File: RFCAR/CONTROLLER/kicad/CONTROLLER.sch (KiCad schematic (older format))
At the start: 6 parts, among them U1 LM1117-3.3, U2 L7805

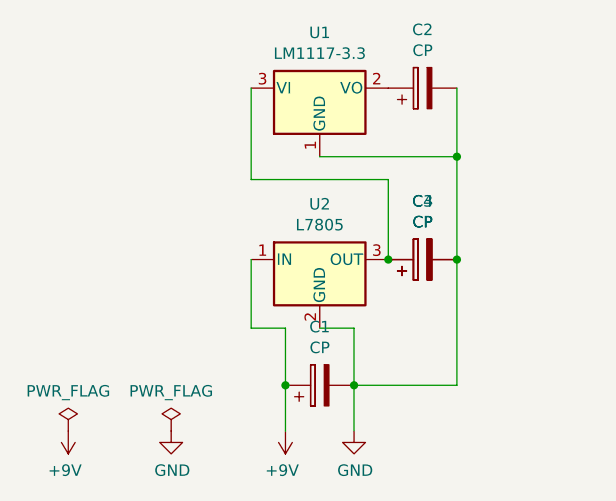
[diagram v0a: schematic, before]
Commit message: kicad
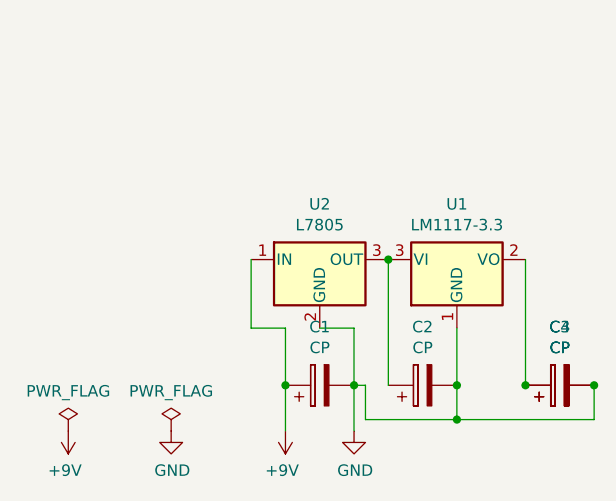
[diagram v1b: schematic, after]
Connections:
- net at U1.3 (VI), U2.3 (OUT): now also C2.1; no longer C3.1, C4.1
- net at U1.2 (VO): now also C3.1, C4.1; no longer C2.1
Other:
- moved on the sheet: C2, C3, C4, U1
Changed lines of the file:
@@
 EESchema Schematic File Version 4
+LIBS:CONTROLLER-cache
 EELAYER 26 0
 EELAYER END
@@
 L Device:CP C3
 U 1 1 5BEC95AE
-P 8050 3950
-F 0 "C3" V 8305 3950 50  0000 C CNN
-F 1 "CP" V 8214 3950 50  0000 C CNN
-F 2 "" H 8088 3800 50  0001 C CNN
-F 3 "~" H 8050 3950 50  0001 C CNN
-	1    8050 3950
+P 8650 4500
+F 0 "C3" V 8905 4500 50  0000 C CNN
+F 1 "CP" V 8814 4500 50  0000 C CNN
+F 2 "" H 8688 4350 50  0001 C CNN
+F 3 "~" H 8650 4500 50  0001 C CNN
+	1    8650 4500
 	0    -1   -1   0
 $EndComp
-Wire Wire Line
-	7750 4500 8200 4500
-Wire Wire Line
-	8200 4500 8200 3950
 $Comp
 L Regulator_Linear:LM1117-3.3 U1
 U 1 1 5BEC973C
-P 7600 3200
-F 0 "U1" H 7600 3442 50  0000 C CNN
-F 1 "LM1117-3.3" H 7600 3351 50  0000 C CNN
-F 2 "" H 7600 3200 50  0001 C CNN
-F 3 "http://www.ti.com/lit/ds/symlink/lm1117.pdf" H 7600 3200 50  0001 C CNN
-	1    7600 3200
+P 8200 3950
+F 0 "U1" H 8200 4192 50  0000 C CNN
+F 1 "LM1117-3.3" H 8200 4101 50  0000 C CNN
+F 2 "" H 8200 3950 50  0001 C CNN
+F 3 "http://www.ti.com/lit/ds/symlink/lm1117.pdf" H 8200 3950 50  0001 C CNN
+	1    8200 3950
 	1    0    0    -1
 $EndComp
@@
 L Device:CP C4
 U 1 1 5BEC976A
-P 8050 3950
-F 0 "C4" V 8305 3950 50  0000 C CNN
-F 1 "CP" V 8214 3950 50  0000 C CNN
-F 2 "" H 8088 3800 50  0001 C CNN
-F 3 "~" H 8050 3950 50  0001 C CNN
-	1    8050 3950
+P 8650 4500
+F 0 "C4" V 8905 4500 50  0000 C CNN
+F 1 "CP" V 8814 4500 50  0000 C CNN
+F 2 "" H 8688 4350 50  0001 C CNN
+F 3 "~" H 8650 4500 50  0001 C CNN
+	1    8650 4500
 	0    -1   -1   0
 $EndComp
-Connection ~ 8200 3950
-Connection ~ 7900 3950
 $Comp
 L Device:CP C2
 U 1 1 5BEC9820
-P 8050 3200
-F 0 "C2" V 8305 3200 50  0000 C CNN
-F 1 "CP" V 8214 3200 50  0000 C CNN
-F 2 "" H 8088 3050 50  0001 C CNN
-F 3 "~" H 8050 3200 50  0001 C CNN
-	1    8050 3200
+P 8050 4500
+F 0 "C2" V 8305 4500 50  0000 C CNN
+F 1 "CP" V 8214 4500 50  0000 C CNN
+F 2 "" H 8088 4350 50  0001 C CNN
+F 3 "~" H 8050 4500 50  0001 C CNN
+	1    8050 4500
 	0    -1   -1   0
 $EndComp
 Wire Wire Line
-	8200 3950 8200 3500
+	7900 3950 7900 4500
 Wire Wire Line
-	8200 3500 7600 3500
+	8200 4250 8200 4500
 Wire Wire Line
-	8200 3500 8200 3200
-Connection ~ 8200 3500
+	7750 4500 7800 4500
 Wire Wire Line
-	7900 3950 7900 3600
+	7800 4500 7800 4650
 Wire Wire Line
-	7900 3600 7300 3600
+	7800 4650 8200 4650
 Wire Wire Line
-	7300 3600 7300 3200
+	8200 4650 8200 4500
+Connection ~ 8200 4500
+Connection ~ 7900 3950
+Wire Wire Line
+	8500 3950 8500 4500
+Connection ~ 8500 4500
+Wire Wire Line
+	8200 4650 8800 4650
+Wire Wire Line
+	8800 4650 8800 4500
+Connection ~ 8200 4650
+Connection ~ 8800 4500
 $EndSCHEMATC
